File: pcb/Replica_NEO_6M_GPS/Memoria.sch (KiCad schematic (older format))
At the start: 2 parts, among them U3 24AA32A-I_MS

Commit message: se hicieron correcciones
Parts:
- U3: footprint SOP65P490X110-8N -> 24AA32A-I_MS:SOP65P490X110-8N
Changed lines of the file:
@@
 Title "i2C EEPROM SERIAL"
 Date "2021-07-12"
-Rev ""
+Rev "1.0"
 Comp "Christian Canaan Castro Botek UBA - Argentina"
 Comment1 ""
@@
 F 0 "U3" H 5400 4370 50  0000 C CNN
 F 1 "24AA32A-I_MS" H 5400 4279 50  0000 C CNN
-F 2 "SOP65P490X110-8N" H 5400 3500 50  0001 L BNN
+F 2 "24AA32A-I_MS:SOP65P490X110-8N" H 5400 3500 50  0001 L BNN
 F 3 "" H 5400 3500 50  0001 L BNN
 	1    5400 3500

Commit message: Se agregaron footprints y se hicieron correcciones menores
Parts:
- C5: footprint (none) -> Capacitor_SMD:C_0805_2012Metric_Pad1.18x1.45mm_HandSolder
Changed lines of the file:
@@
 F 0 "C5" H 6615 3496 50  0000 L CNN
 F 1 "0.1uF" H 6615 3405 50  0000 L CNN
-F 2 "" H 6538 3300 50  0001 C CNN
+F 2 "Capacitor_SMD:C_0805_2012Metric_Pad1.18x1.45mm_HandSolder" H 6538 3300 50  0001 C CNN
 F 3 "~" H 6500 3450 50  0001 C CNN
 	1    6500 3450

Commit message: Se acomodaron archivos y se hicieron retoques
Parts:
- U3: symbol 24AA32A-I_MS:24AA32A-I_MS -> Replica_NEO_6M_GPS-rescue:24AA32A-I_MS-24AA32A-I_MS
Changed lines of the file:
@@
 $EndDescr
 $Comp
-L 24AA32A-I_MS:24AA32A-I_MS U3
+L Replica_NEO_6M_GPS-rescue:24AA32A-I_MS-24AA32A-I_MS U3
 U 1 1 60EE7965
 P 5400 3500
+AR Path="/60EE7965" Ref="U3"  Part="1"
+AR Path="/60EC55E9/60EE7965" Ref="U3"  Part="1"
 F 0 "U3" H 5400 4370 50  0000 C CNN
 F 1 "24AA32A-I_MS" H 5400 4279 50  0000 C CNN

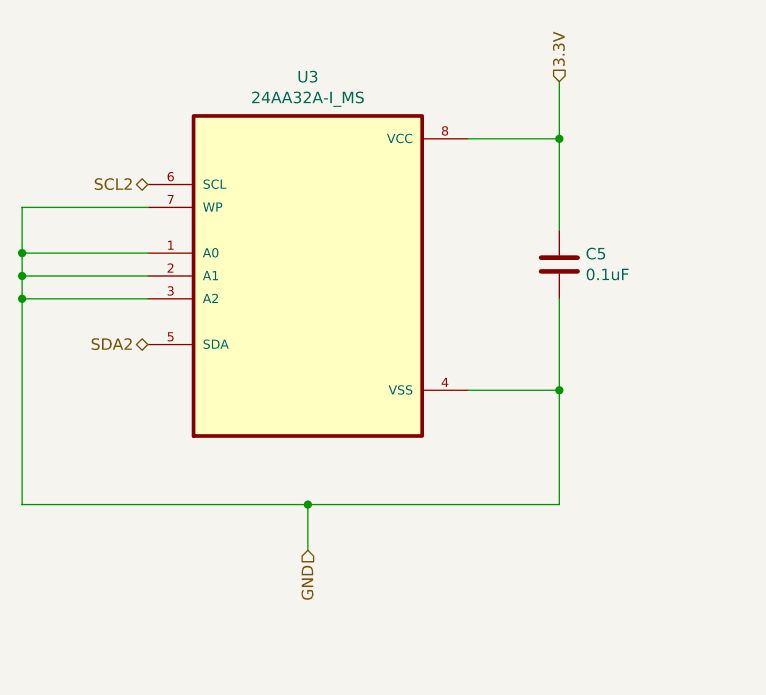
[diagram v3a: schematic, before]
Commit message: se retoco el esquematico
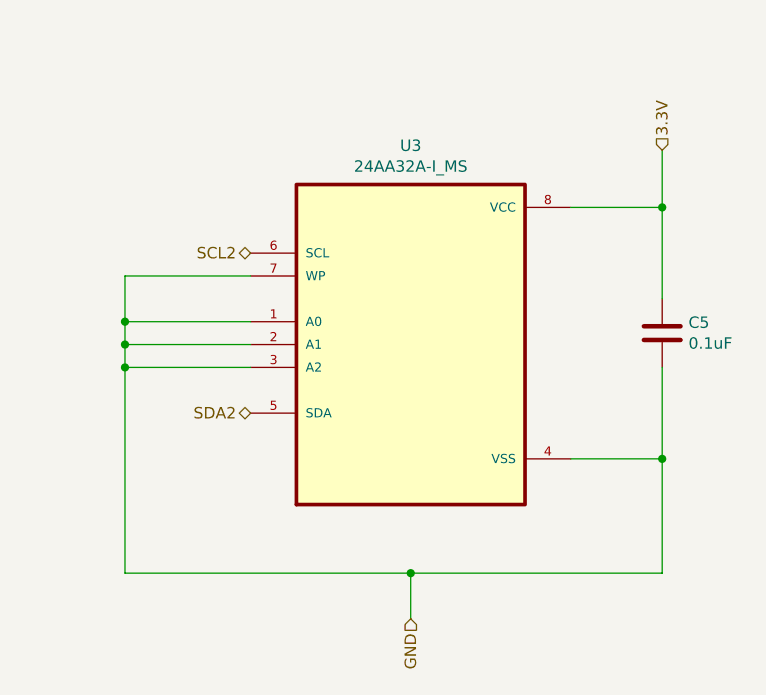
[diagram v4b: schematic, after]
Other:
- moved on the sheet: C5, U3
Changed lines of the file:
@@
 L Replica_NEO_6M_GPS-rescue:24AA32A-I_MS-24AA32A-I_MS U3
 U 1 1 60EE7965
-P 5400 3500
+P 5850 3800
 AR Path="/60EE7965" Ref="U3"  Part="1"
 AR Path="/60EC55E9/60EE7965" Ref="U3"  Part="1"
-F 0 "U3" H 5400 4370 50  0000 C CNN
-F 1 "24AA32A-I_MS" H 5400 4279 50  0000 C CNN
-F 2 "24AA32A-I_MS:SOP65P490X110-8N" H 5400 3500 50  0001 L BNN
-F 3 "" H 5400 3500 50  0001 L BNN
-	1    5400 3500
+F 0 "U3" H 5850 4670 50  0000 C CNN
+F 1 "24AA32A-I_MS" H 5850 4579 50  0000 C CNN
+F 2 "24AA32A-I_MS:SOP65P490X110-8N" H 5850 3800 50  0001 L BNN
+F 3 "" H 5850 3800 50  0001 L BNN
+	1    5850 3800
 	1    0    0    -1
 $EndComp
@@
 L Device:C C5
 U 1 1 60EE920D
-P 6500 3450
-F 0 "C5" H 6615 3496 50  0000 L CNN
-F 1 "0.1uF" H 6615 3405 50  0000 L CNN
-F 2 "Capacitor_SMD:C_0805_2012Metric_Pad1.18x1.45mm_HandSolder" H 6538 3300 50  0001 C CNN
-F 3 "~" H 6500 3450 50  0001 C CNN
-	1    6500 3450
+P 6950 3750
+F 0 "C5" H 7065 3796 50  0000 L CNN
+F 1 "0.1uF" H 7065 3705 50  0000 L CNN
+F 2 "Capacitor_SMD:C_0805_2012Metric_Pad1.18x1.45mm_HandSolder" H 6988 3600 50  0001 C CNN
+F 3 "~" H 6950 3750 50  0001 C CNN
+	1    6950 3750
 	1    0    0    -1
 $EndComp
 Wire Wire Line
-	6500 2900 6500 3300
+	6950 3200 6950 3600
 Wire Wire Line
-	6500 3600 6500 4000
+	6950 3900 6950 4300
 Wire Wire Line
-	6500 4500 5400 4500
+	6950 4800 5850 4800
 Wire Wire Line
-	5400 4500 5400 4700
-Connection ~ 6500 4000
+	5850 4800 5850 5000
+Connection ~ 6950 4300
 Wire Wire Line
-	6500 4000 6500 4500
+	6950 4300 6950 4800
 Wire Wire Line
-	4150 3200 4150 3400
-Connection ~ 5400 4500
-Connection ~ 4150 3400
+	4600 3500 4600 3700
+Connection ~ 5850 4800
+Connection ~ 4600 3700
 Wire Wire Line
-	4150 3400 4150 3500
-Connection ~ 4150 3500
+	4600 3700 4600 3800
+Connection ~ 4600 3800
 Wire Wire Line
-	4150 3500 4150 3600
-Connection ~ 4150 3600
+	4600 3800 4600 3900
+Connection ~ 4600 3900
 Wire Wire Line
-	4150 3600 4150 4500
+	4600 3900 4600 4800
 Wire Wire Line
-	6500 2650 6500 2900
-Connection ~ 6500 2900
+	6950 2950 6950 3200
+Connection ~ 6950 3200
 Wire Wire Line
-	6100 2900 6500 2900
+	6550 3200 6950 3200
 Wire Wire Line
-	6100 4000 6500 4000
+	6550 4300 6950 4300
 Wire Wire Line
-	4150 3200 4700 3200
+	4600 3500 5150 3500
 Wire Wire Line
-	4150 3400 4700 3400
+	4600 3700 5150 3700
 Wire Wire Line
-	4150 3500 4700 3500
+	4600 3800 5150 3800
 Wire Wire Line
-	4150 3600 4700 3600
+	4600 3900 5150 3900
 Wire Wire Line
-	4150 4500 5400 4500
-Text HLabel 5400 4700 3    50   Input ~ 0
+	4600 4800 5850 4800
+Text HLabel 5850 5000 3    50   Input ~ 0
 GND
-Text HLabel 4700 3100 0    50   BiDi ~ 0
+Text HLabel 5150 3400 0    50   BiDi ~ 0
 SCL2
-Text HLabel 4700 3800 0    50   BiDi ~ 0
+Text HLabel 5150 4100 0    50   BiDi ~ 0
 SDA2
-Text HLabel 6500 2650 1    50   Input ~ 0
+Text HLabel 6950 2950 1    50   Input ~ 0
 3.3V
 $EndSCHEMATC
